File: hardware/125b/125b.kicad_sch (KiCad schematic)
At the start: 51 parts, among them J1 Guitar in, J2 Barrel_Jack, J3 Conn_02x05_Odd_Even_MountingP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, J4 Guitar out, SW1 SW_DIP_x02, SW2 RotaryEncoder_Switch, SW3 Switch 1, SW4 Switch 2, U1 L78L05_TO92, U2 TL074

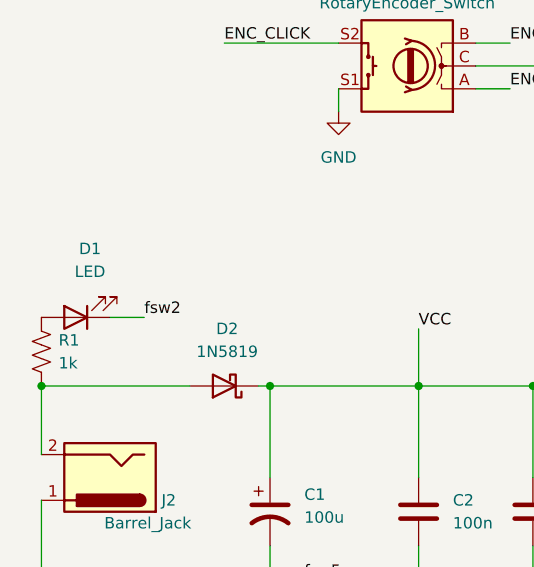
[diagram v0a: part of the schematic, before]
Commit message: Everything connected together
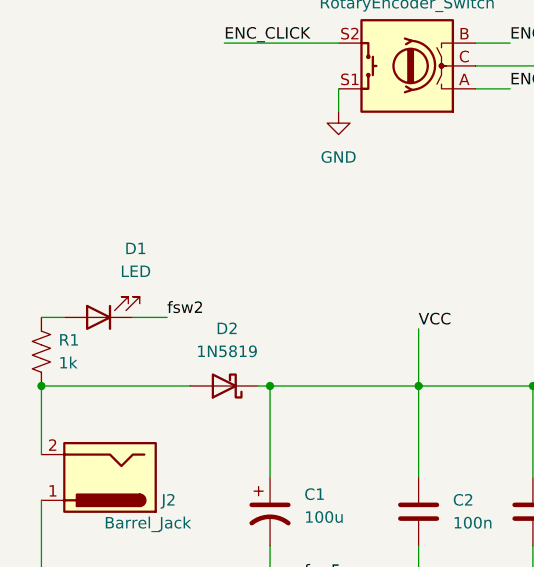
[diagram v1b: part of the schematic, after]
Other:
- moved on the sheet: D1
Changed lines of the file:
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@@
 	(wire
 		(pts
-			(xy 26.67 153.67) (xy 30.48 153.67)
+			(xy 29.21 153.67) (xy 33.02 153.67)
 		)
 		(stroke
@@
 	(wire
 		(pts
+			(xy 19.05 153.67) (xy 21.59 153.67)
+		)
+		(stroke
+			(width 0)
+			(type default)
+		)
+	)
+	(wire
+		(pts
 			(xy 133.35 52.07) (xy 148.59 52.07)
 		)
@@
 	)
 	(label "fsw2"
-		(at 30.48 153.67 0)
+		(at 33.02 153.67 0)
 		(effects
 			(font
@@
 		)
 	)
+	(netclass_flag ""
+		(length 2.54)
+		(shape round)
+		(at 53.34 161.29 0)
+		(fields_autoplaced yes)
+		(effects
+			(font
+				(size 1.27 1.27)
+			)
+			(justify left bottom)
+		)
+		(property "Netclass" "Power"
+			(at 54.0385 158.75 0)
+			(effects
+				(font
+					(size 1.27 1.27)
+				)
+				(justify left)
+			)
+		)
+		(property "Component Class" ""
+			(at 1.27 1.27 0)
+			(effects
+				(font
+					(size 1.27 1.27)
+					(italic yes)
+				)
+			)
+		)
+	)
+	(netclass_flag ""
+		(length 2.54)
+		(shape round)
+		(at 111.76 161.29 0)
+		(fields_autoplaced yes)
+		(effects
+			(font
+				(size 1.27 1.27)
+			)
+			(justify left bottom)
+		)
+		(property "Netclass" "Power"
+			(at 112.4585 158.75 0)
+			(effects
+				(font
+					(size 1.27 1.27)
+				)
+				(justify left)
+			)
+		)
+		(property "Component Class" ""
+			(at -1.27 0 0)
+			(effects
+				(font
+					(size 1.27 1.27)
+					(italic yes)
+				)
+			)
+		)
+	)
+	(netclass_flag ""
+		(length 2.54)
+		(shape round)
+		(at 31.75 153.67 0)
+		(fields_autoplaced yes)
+		(effects
+			(font
+				(size 1.27 1.27)
+			)
+			(justify left bottom)
+		)
+		(property "Netclass" "Power"
+			(at 32.4485 151.13 0)
+			(effects
+				(font
+					(size 1.27 1.27)
+				)
+				(justify left)
+			)
+		)
+		(property "Component Class" ""
+			(at -45.72 8.89 0)
+			(effects
+				(font
+					(size 1.27 1.27)
+					(italic yes)
+				)
+			)
+		)
+	)
+	(netclass_flag ""
+		(length 2.54)
+		(shape round)
+		(at 20.32 153.67 0)
+		(fields_autoplaced yes)
+		(effects
+			(font
+				(size 1.27 1.27)
+			)
+			(justify left bottom)
+		)
+		(property "Netclass" "Power"
+			(at 21.0185 151.13 0)
+			(effects
+				(font
+					(size 1.27 1.27)
+				)
+				(justify left)
+			)
+		)
+		(property "Component Class" ""
+			(at -57.15 8.89 0)
+			(effects
+				(font
+					(size 1.27 1.27)
+					(italic yes)
+				)
+			)
+		)
+	)
+	(netclass_flag ""
+		(length 2.54)
+		(shape round)
+		(at 27.94 161.29 0)
+		(fields_autoplaced yes)
+		(effects
+			(font
+				(size 1.27 1.27)
+			)
+			(justify left bottom)
+		)
+		(property "Netclass" "Power"
+			(at 28.6385 158.75 0)
+			(effects
+				(font
+					(size 1.27 1.27)
+				)
+				(justify left)
+			)
+		)
+		(property "Component Class" ""
+			(at -168.91 17.78 0)
+			(effects
+				(font
+					(size 1.27 1.27)
+					(italic yes)
+				)
+			)
+		)
+	)
 	(symbol
 		(lib_name "GND_15")
@@
 	(symbol
 		(lib_id "Device:LED")
-		(at 22.86 153.67 180)
+		(at 25.4 153.67 180)
 		(unit 1)
 		(exclude_from_sim no)
@@
 		(on_board yes)
 		(dnp no)
-		(fields_autoplaced yes)
 		(property "Reference" "D1"
-			(at 24.4475 146.05 0)
+			(at 29.5275 146.05 0)
 			(effects
 				(font
@@
 		)
 		(property "Value" "LED"
-			(at 24.4475 148.59 0)
+			(at 29.5275 148.59 0)
 			(effects
 				(font
@@
 		)
 		(property "Footprint" "LED_THT:LED_D1.8mm_W3.3mm_H2.4mm"
-			(at 22.86 153.67 0)
+			(at 25.4 153.67 0)
 			(effects
 				(font
@@
 		)
 		(property "Datasheet" "~"
-			(at 22.86 153.67 0)
+			(at 25.4 153.67 0)
 			(effects
 				(font
@@
 		)
 		(property "Description" "Light emitting diode"
-			(at 22.86 153.67 0)
+			(at 25.4 153.67 0)
 			(effects
 				(font
@@
 		)
 		(property "Sim.Pins" "1=K 2=A"
-			(at 22.86 153.67 0)
+			(at 25.4 153.67 0)
 			(effects
 				(font
